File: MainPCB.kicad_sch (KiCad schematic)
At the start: 41 parts, among them J1 RaspberryPi, J10 Conn_01x02, J2 Conn_01x03, J3 Screw_Terminal_01x02, J4 Conn_01x02, J5 Conn_01x06, J6 Conn_01x03_Pin, J7 Conn_01x10, J8 Conn_01x12, J9 Conn_01x04, M1 Motor_DC, M2 Motor_DC, M3 Motor_DC, M4 Motor_DC, SW1 SW_SPDT, SW2 SW_SPDT, SW3 SW_SPDT, SW4 SW_SPDT, SW5 SW_SPDT, SW6 SW_SPDT, SW7 SW_SPDT, U1 Teensy4.1, U10 Compass, U11 V_Regulator5v, U12 RockerSwitch, U13 V_Regulator3.3v, U2 VNH Driver, U3 VNH Driver, U4 VNH Driver, U5 VNH Driver, U6 TSOP25xx

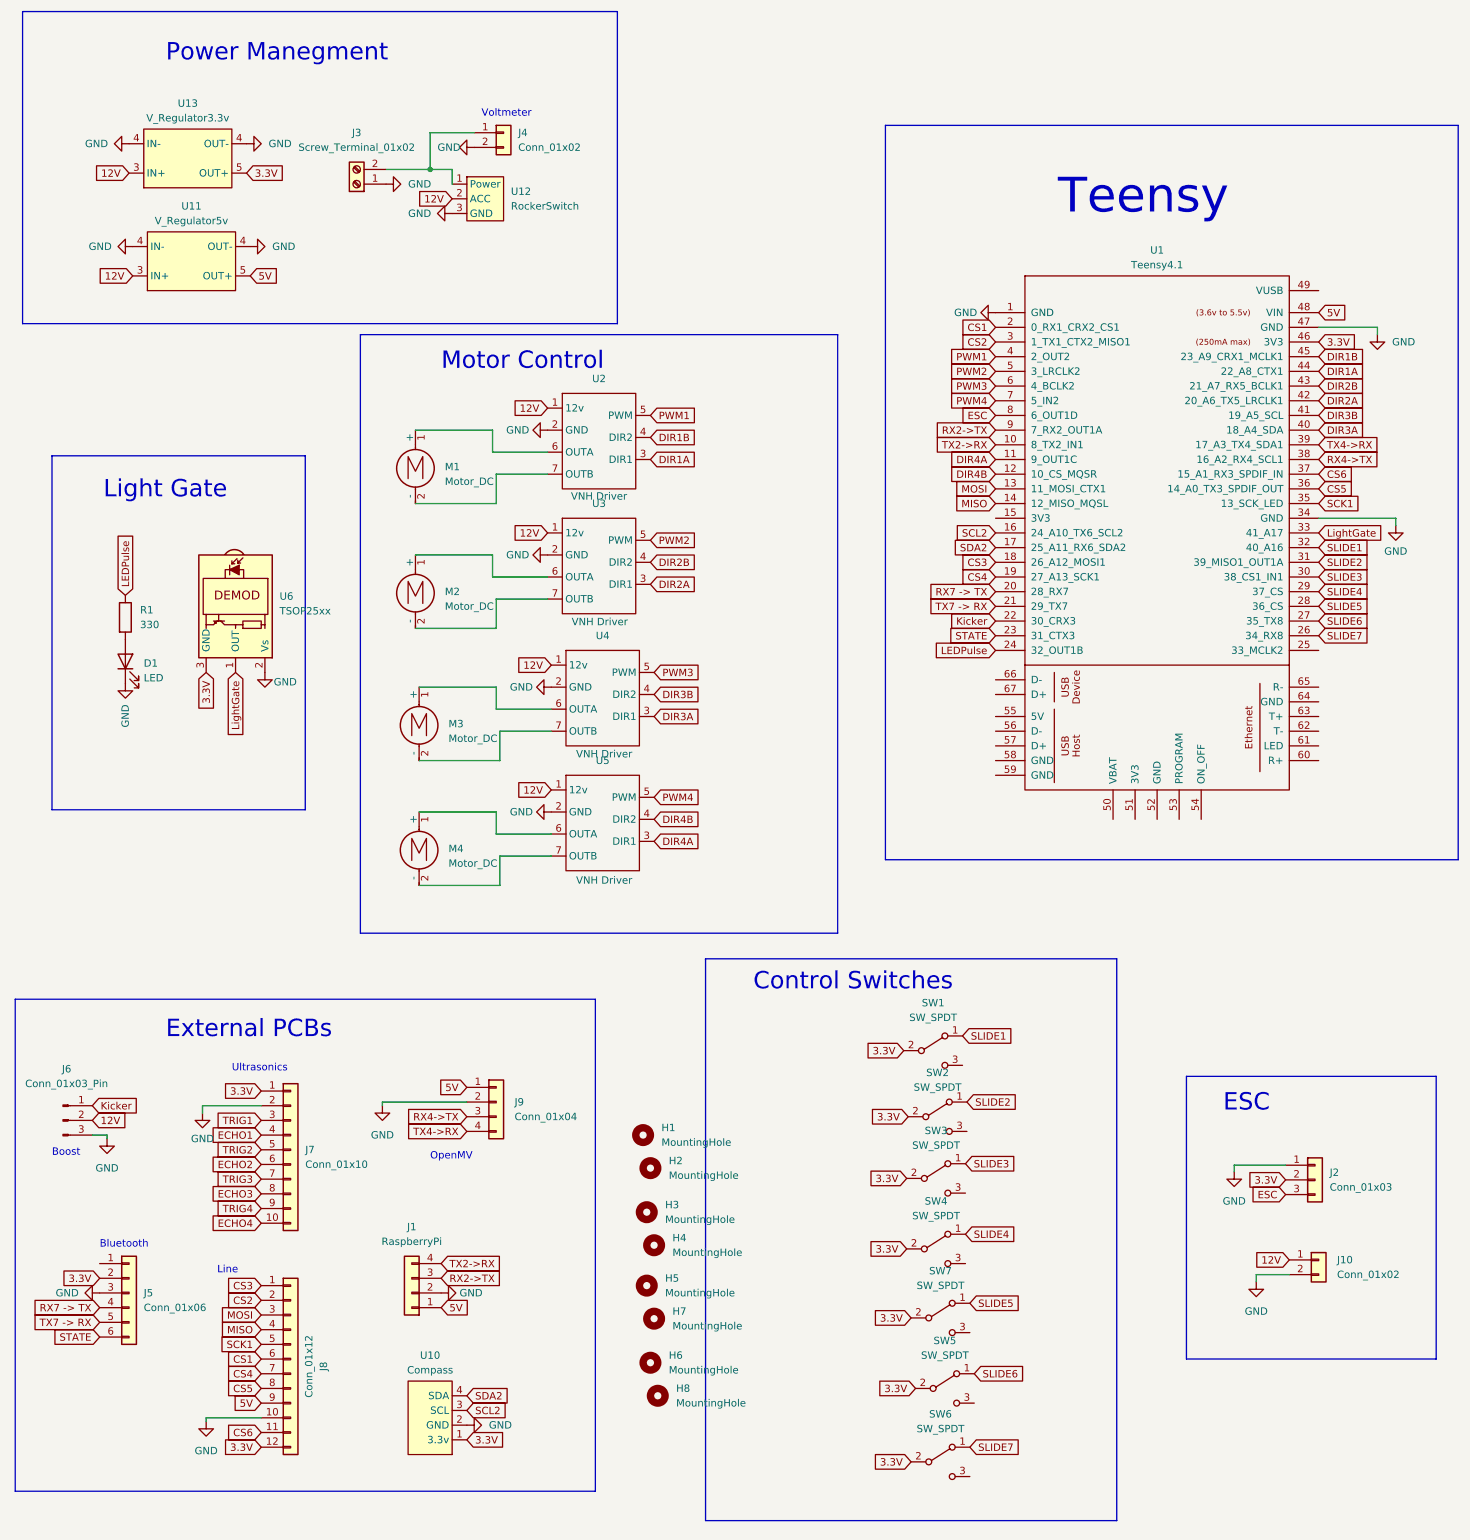
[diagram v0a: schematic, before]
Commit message: Finshined again
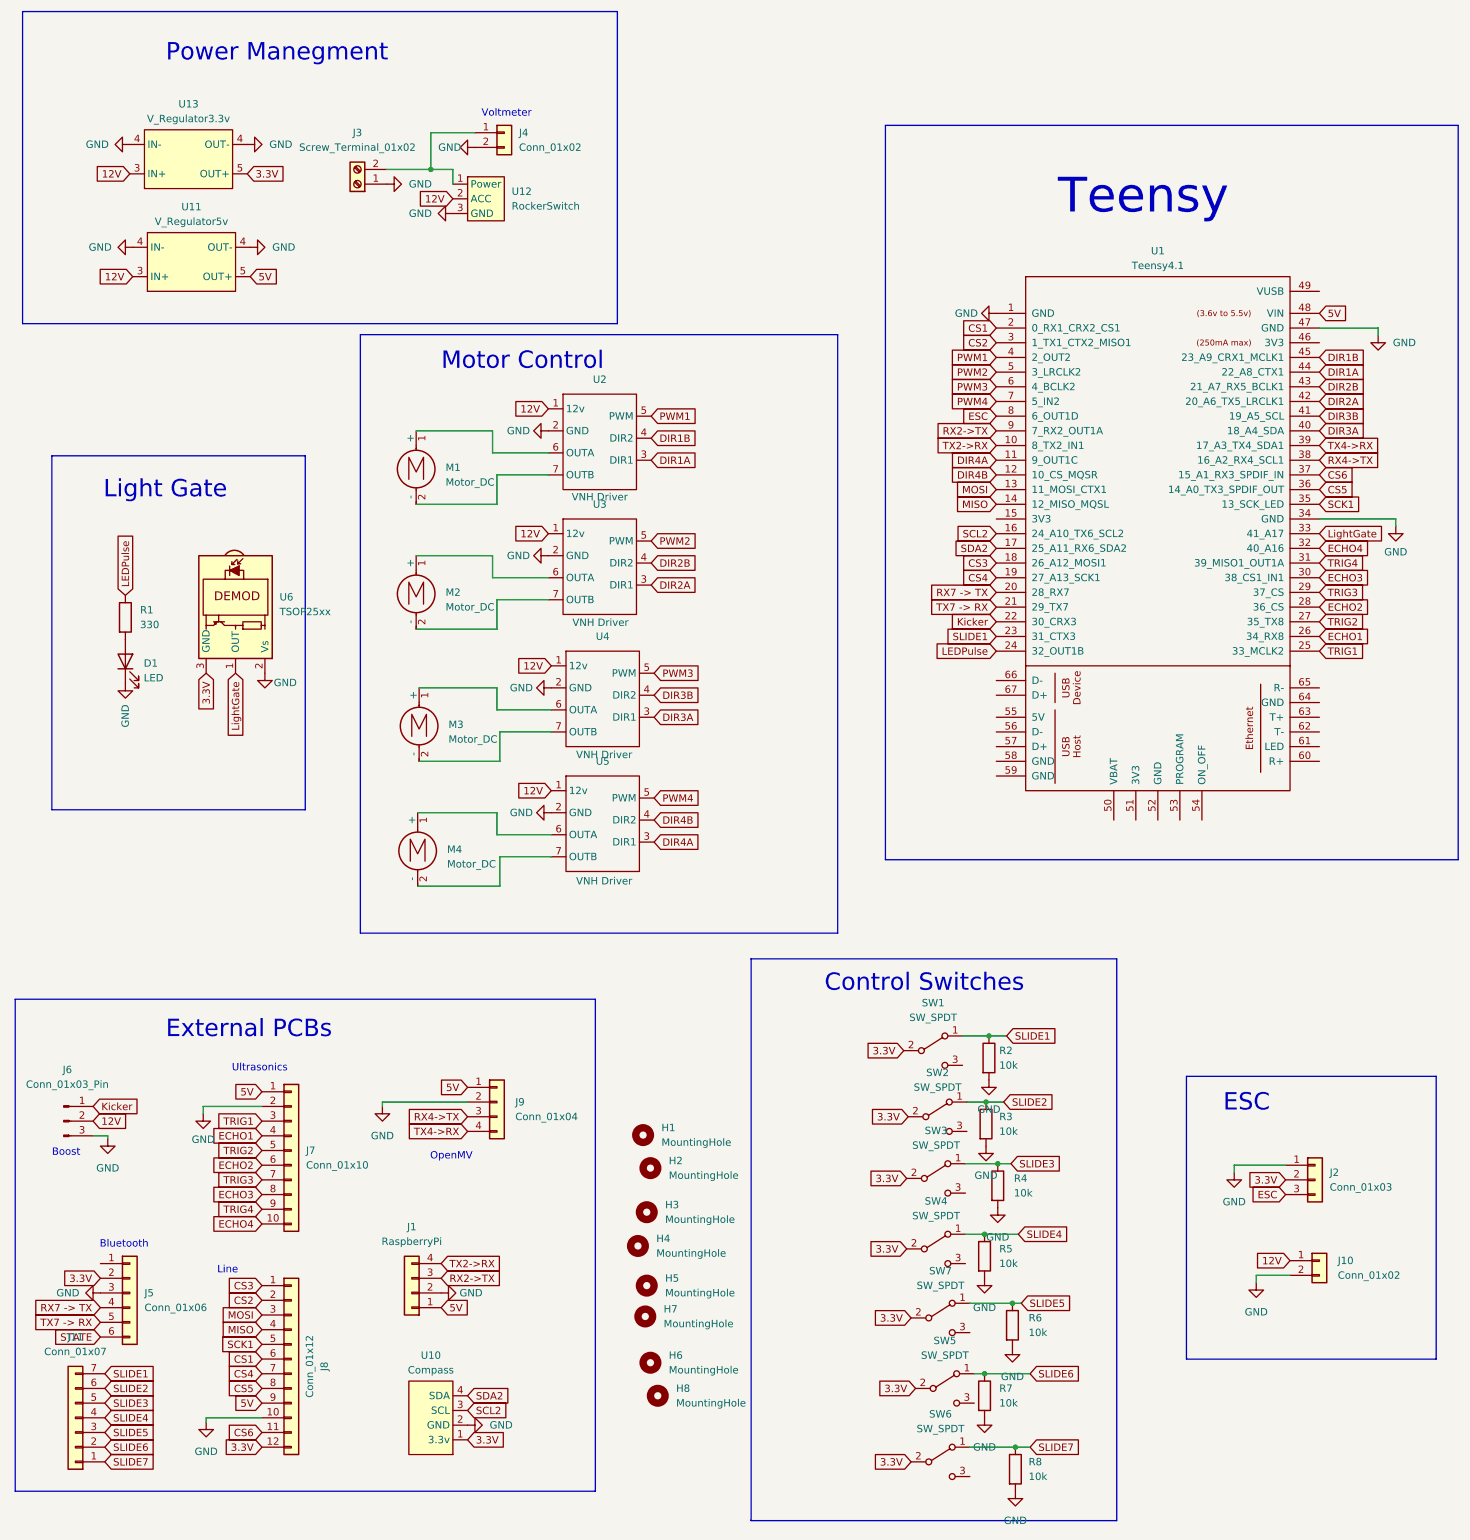
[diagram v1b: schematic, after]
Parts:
- added J11: Conn_01x07, Connector_PinHeader_2.54mm:PinHeader_1x07_P2.54mm_Vertical, symbol Connector_Generic:Conn_01x07
- added R2, R3, R4, R5, R6, R7, R8: 10k, Capacitor_SMD:C_0805_2012Metric_Pad1.18x1.45mm_HandSolder, symbol Device:R
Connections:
- net 3.3V: no longer J7.1 (Pin_1), U1.46 (3V3)
- net 5V: now also J7.1 (Pin_1)
- net ECHO1: now also U1.26 (34_RX8)
- net ECHO2: now also U1.28 (36_CS)
- net ECHO3: now also U1.30 (38_CS1_IN1)
- net ECHO4: now also U1.32 (40_A16)
- net GND: now also R2.2, R3.2, R4.2, R5.2, R6.2, R7.2, R8.2
- net SLIDE1: now also U1.23 (31_CTX3), J11.7 (Pin_7), R2.1; no longer U1.32 (40_A16)
- net SLIDE2: now also J11.6 (Pin_6), R3.1; no longer U1.31 (39_MISO1_OUT1A)
- net SLIDE3: now also J11.5 (Pin_5), R4.1; no longer U1.30 (38_CS1_IN1)
- net SLIDE4: now also J11.4 (Pin_4), R5.1; no longer U1.29 (37_CS)
- net SLIDE5: now also J11.3 (Pin_3), R6.1; no longer U1.28 (36_CS)
- net SLIDE6: now also J11.2 (Pin_2), R7.1; no longer U1.27 (35_TX8)
- net SLIDE7: now also J11.1 (Pin_1), R8.1; no longer U1.26 (34_RX8)
- net STATE: no longer U1.23 (31_CTX3)
- net TRIG1: now also U1.25 (33_MCLK2)
- net TRIG2: now also U1.27 (35_TX8)
- net TRIG3: now also U1.29 (37_CS)
- net TRIG4: now also U1.31 (39_MISO1_OUT1A)
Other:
- moved on the sheet: H4, H7

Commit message: part movement
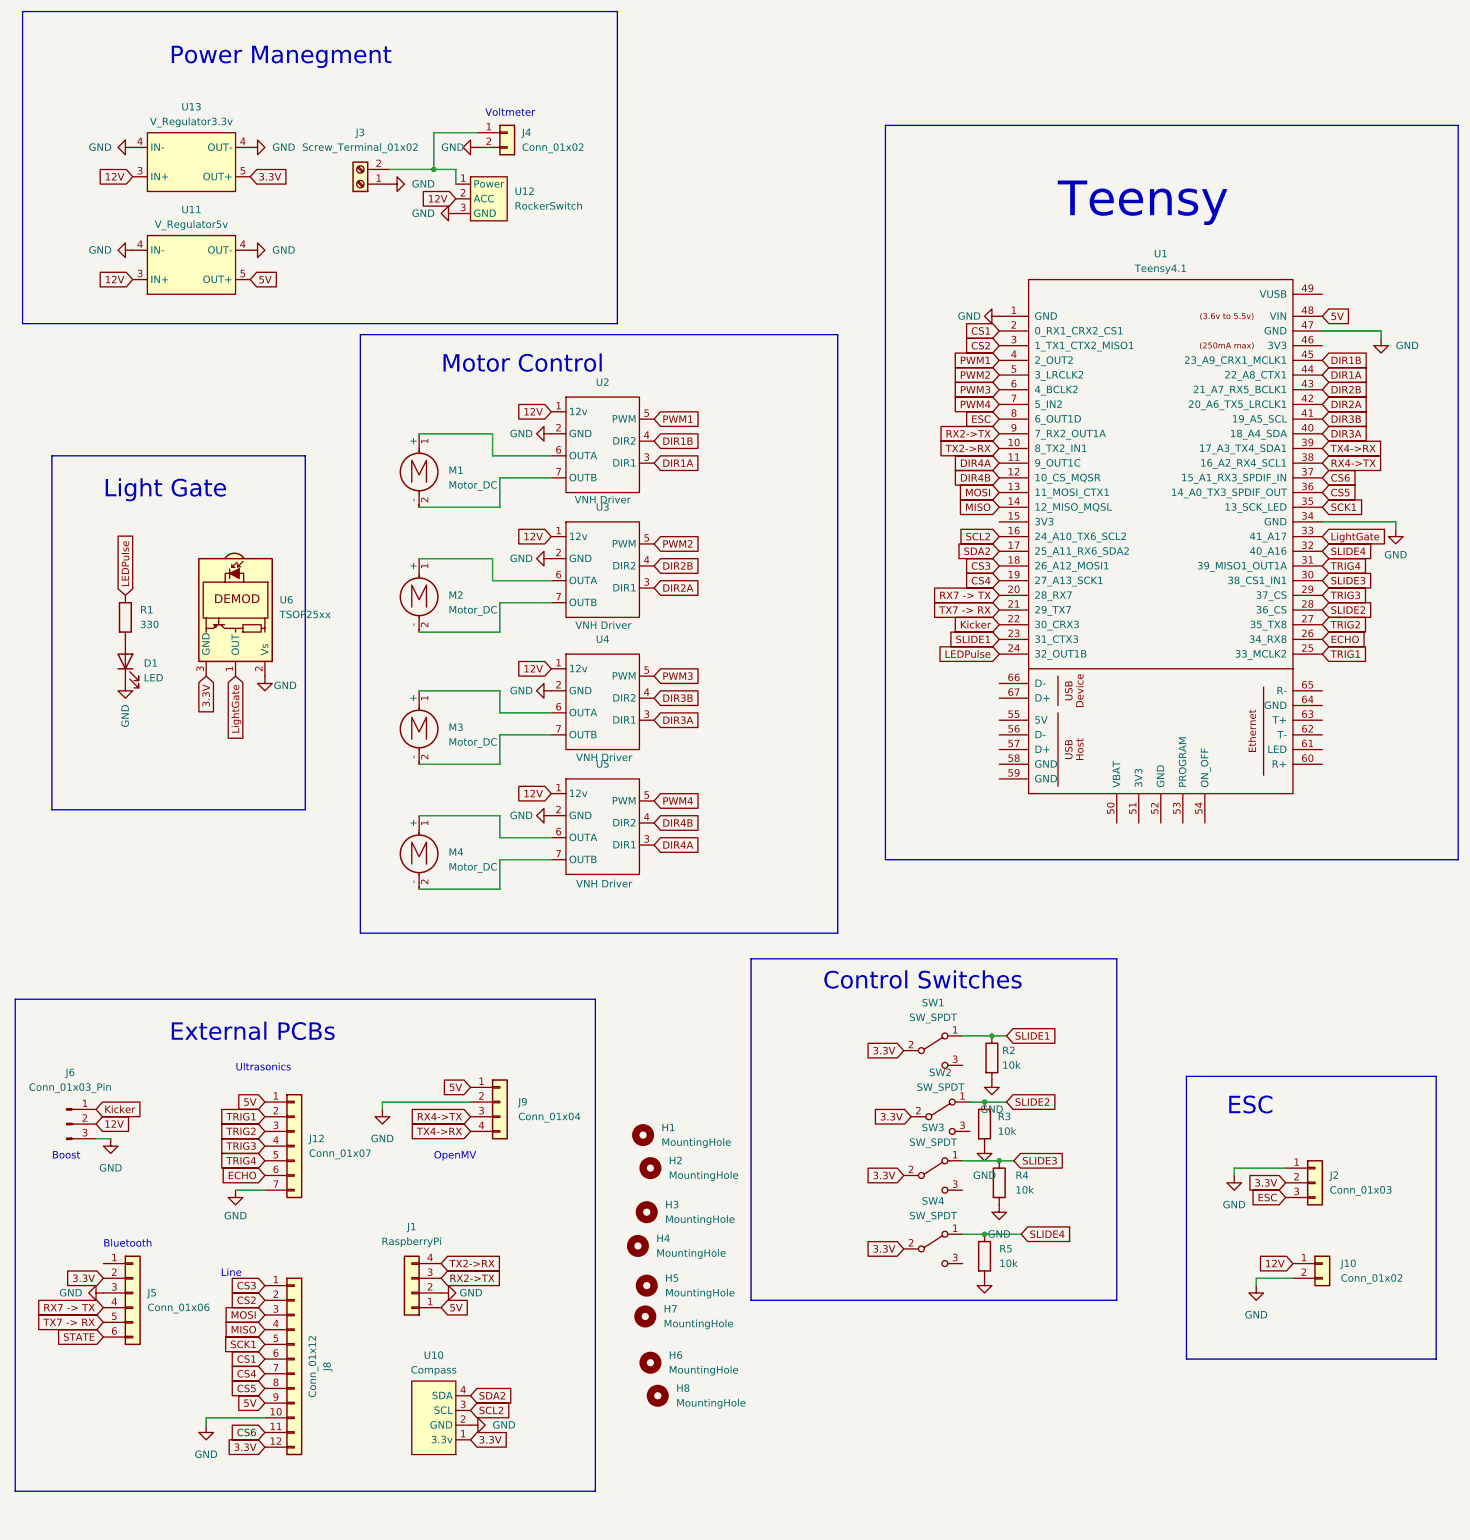
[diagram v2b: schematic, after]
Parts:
- removed J11: Conn_01x07, Connector_PinHeader_2.54mm:PinHeader_1x07_P2.54mm_Vertical, symbol Connector_Generic:Conn_01x07
- removed J7: Conn_01x10, Connector_IDC:IDC-Header_2x05_P2.54mm_Vertical, symbol Connector_Generic:Conn_01x10
- removed R6, R7, R8: 10k, Capacitor_SMD:C_0805_2012Metric_Pad1.18x1.45mm_HandSolder, symbol Device:R
- removed SW5, SW6, SW7: SW_SPDT, SlideSW:SPDT_OS102011_CNK, symbol Switch:SW_SPDT
- added J12: Conn_01x07, Connector_IDC:IDC-Header_2x04_P2.54mm_Vertical, symbol Connector_Generic:Conn_01x07
- H1, H2, H3, H4: footprint MountingHole:MountingHole_3.2mm_M3 -> MountingHole:MountingHole_3.2mm_M3_DIN965_Pad
- H5, H6, H7, H8: footprint MountingHole:MountingHole_2.7mm_M2.5 -> MountingHole:MountingHole_2.7mm_M2.5_DIN965_Pad
- U10: footprint Connector_PinHeader_2.54mm:PinHeader_1x04_P2.54mm_Vertical -> Custom:Compass Sensor DFRobot
- U11, U13: footprint Connector_PinHeader_2.54mm:PinHeader_1x05_P2.54mm_Vertical -> Custom:Pololu Regulator
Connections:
- net ECHO2 is gone; now on net SLIDE2: U1.28 (36_CS)
- net ECHO3 is gone; now on net SLIDE3: U1.30 (38_CS1_IN1)
- net ECHO4 is gone; now on net SLIDE4: U1.32 (40_A16)
- net 5V: now also J12.1 (Pin_1)
- net GND: now also J12.7 (Pin_7)
- net TRIG1: now also J12.2 (Pin_2)
- net TRIG2: now also J12.3 (Pin_3)
- net TRIG3: now also J12.4 (Pin_4)
- net TRIG4: now also J12.5 (Pin_5)
- net ECHO1 renamed ECHO
- net ECHO: now also J12.6 (Pin_6)
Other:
- moved on the sheet: J10, J2, J3, J4, J5, J6, J8, J9, M1, M2, M3, M4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

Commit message: Made Changes
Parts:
- H5, H6, H7, H8: footprint MountingHole:MountingHole_2.7mm_M2.5_DIN965_Pad -> MountingHole:MountingHole_3.2mm_M3_DIN965_Pad
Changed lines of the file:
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@@
 			)
 		)
-		(property "Footprint" "MountingHole:MountingHole_2.7mm_M2.5_DIN965_Pad"
+		(property "Footprint" "MountingHole:MountingHole_3.2mm_M3_DIN965_Pad"
 			(at 127.635 256.54 0)
 			(effects
@@
 			)
 		)
-		(property "Footprint" "MountingHole:MountingHole_2.7mm_M2.5_DIN965_Pad"
+		(property "Footprint" "MountingHole:MountingHole_3.2mm_M3_DIN965_Pad"
 			(at 125.73 237.49 0)
 			(effects
@@
 			)
 		)
-		(property "Footprint" "MountingHole:MountingHole_2.7mm_M2.5_DIN965_Pad"
+		(property "Footprint" "MountingHole:MountingHole_3.2mm_M3_DIN965_Pad"
 			(at 126.365 250.825 0)
 			(effects
@@
 			)
 		)
-		(property "Footprint" "MountingHole:MountingHole_2.7mm_M2.5_DIN965_Pad"
+		(property "Footprint" "MountingHole:MountingHole_3.2mm_M3_DIN965_Pad"
 			(at 125.476 242.824 0)
 			(effects
